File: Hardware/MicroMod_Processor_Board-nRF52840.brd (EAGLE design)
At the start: 22 x 22 mm, 29 parts, among them J1 MICROMOD-2222, U1 W25QXX128MBIT-6X5, U2 MDBT50Q, Y1 32.768kHz

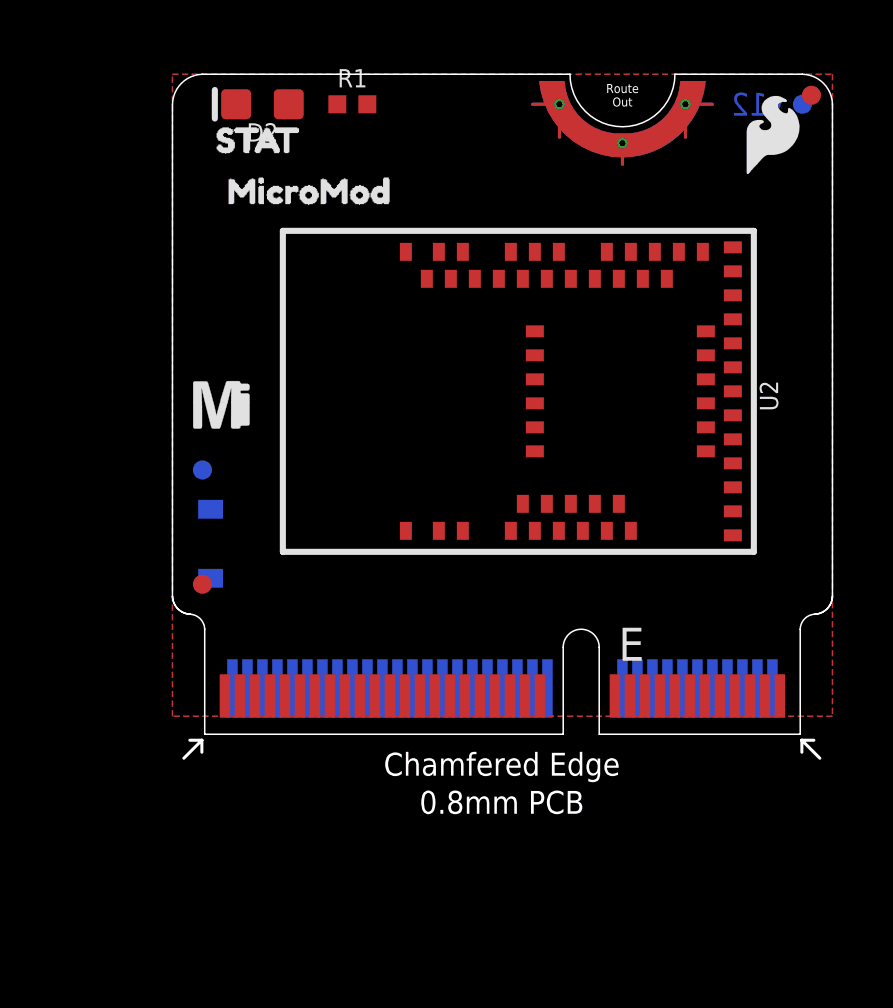
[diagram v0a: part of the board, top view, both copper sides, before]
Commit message: Working on schematic
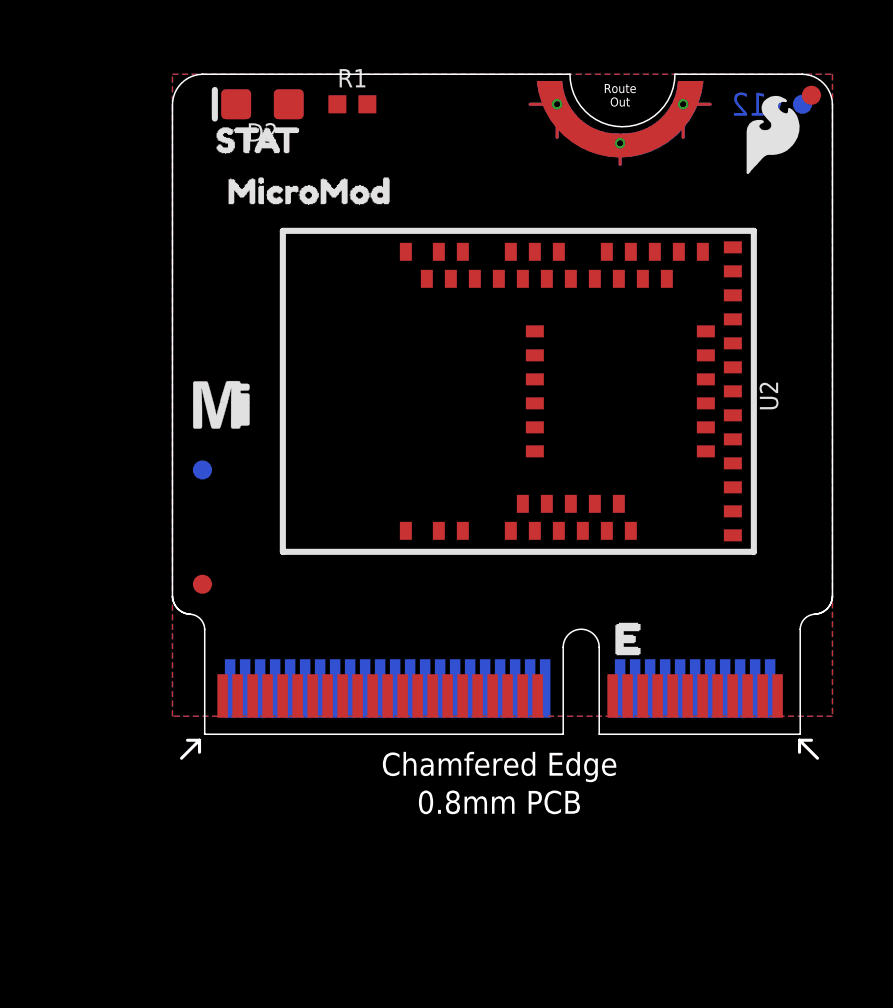
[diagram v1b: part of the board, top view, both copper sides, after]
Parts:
- removed D7: 1A/23V/620mV, SparkFun-DiscreteSemi:SOD-323
- removed J1: MICROMOD-2222, SparkFun-MicroMod:M.2-CARD-E-22
- added J2: MICROMOD-2222, SparkFun-MicroMod:M.2-CARD-E-22
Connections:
- removed net 3.3V_MAIN: D7.A, J1.2, J1.74
- removed net CAM_PCLK: J1.54
- removed net CLKOUT: J1.56, J1.58
- new net N$6: U1.1
- new net USB_VIN: J2.9, U2.32
- net !RESET!: now also J2.6; no longer J1.6
- net 3.3V: now also J2.2, J2.74; no longer D7.C, J1.72
- net 3.3V_EN: now also J2.4; no longer J1.4
- net ADC0: now also J2.34, U2.20; no longer J1.34
- net ADC1: now also J2.38, U2.21; no longer J1.38
- net ADC_D+: now also J2.63, U2.13; no longer J1.63
- net ADC_D-: now also J2.65, U2.11; no longer J1.65
- net BATT_VIN/3: now also J2.49, U2.10; no longer J1.51
- net BOOT: now also J2.11; no longer J1.11
- net CTS1: now also J2.15, U2.22; no longer J1.15
- net D0: now also J2.10, U2.16; no longer J1.10
- net D1: now also J2.18, U2.25; no longer J1.18
- net GND: now also J2.1, J2.33, J2.36, J2.39, J2.45, J2.7, J2.75, J2.GND1, J2.GND2, J2.GND3; no longer J1.1, J1.33, J1.36, J1.39, J1.45, J1.7, J1.75, J1.GND1, J1.GND2, J1.GND3
- net GPIO0: now also J2.40, U2.8; no longer J1.40, U2.57
- net GPIO1: now also J2.42, U2.7; no longer J1.42, U2.58
- net GPIO2: now also J2.44, U2.6; no longer J1.44, U2.25
- net GPIO3: now also J2.46, U2.5; no longer J1.46, U2.26
- net GPIO4: now also J2.48, U2.4; no longer J1.48, U2.3
- net GPIO5: now also J2.73, U2.3; no longer J1.73, U2.4
- net GPIO6: now also J2.71, U2.57; no longer J1.71, U2.5
- net GPIO7: now also J2.69, U2.56; no longer J1.69, U2.6
- net I2C_!INT!: now also J2.16, U2.60; no longer J1.16
- net NFC1: now also J2.43; no longer J1.43
- net NFC2: now also J2.41; no longer J1.41
- net PDM_CLK: now also J2.50, U2.49; no longer J1.50
- net PDM_DATA: now also J2.52, U2.50; no longer J1.52
- net PWM0: now also J2.32, U2.26; no longer J1.32
- net PWM1: now also J2.47, U2.38; no longer J1.47
- net RTS1: now also J2.13, U2.19; no longer J1.13
- net RX1: now also J2.19; no longer J1.19
- net RX2: now also J2.20, U2.59; no longer J1.20, U2.42
- net SCL: now also J2.14; no longer J1.14
- net SCL1: now also J2.53, U2.48; no longer J1.55
- net SDA: now also J2.12; no longer J1.12
- net SDA1: now also J2.51, U2.61; no longer J1.53
- net SDIO_DATA1: now also J2.66, U1.2, U2.46; no longer J1.66, U2.60
- net SDIO_DATA2: now also J2.68, U1.3, U2.45; no longer J1.68, U2.56
- net SPI_!CS!: now also J2.70, U1.7, U2.47; no longer J1.70, U2.59
- net SPI_!CS!1: now also J2.55, U2.44; no longer J1.49
- net SPI_MISO: now also J2.64, U1.5, U2.43; no longer J1.64, U2.50
- net SPI_MISO1: now also J2.61; no longer J1.61
- net SPI_MOSI: now also J2.62, U2.40; no longer J1.62, U2.61
- net SPI_MOSI1: now also J2.59; no longer J1.59
- net SPI_SCK: now also J2.60, U1.6, U2.42; no longer J1.60, U2.47
- net SPI_SCK1: now also J2.57; no longer J1.57
- net SWDCK: now also J2.21; no longer J1.21
- net SWDIO: now also J2.23; no longer J1.23
- net TX1: now also J2.17; no longer J1.17
- net TX2: now also J2.22, U2.58; no longer J1.22, U2.44
- net USB_D+: now also J2.3; no longer J1.3
- net USB_D-: now also J2.5; no longer J1.5
